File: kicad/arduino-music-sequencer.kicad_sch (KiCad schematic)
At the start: 130 parts, among them U1 CD74HC4067M

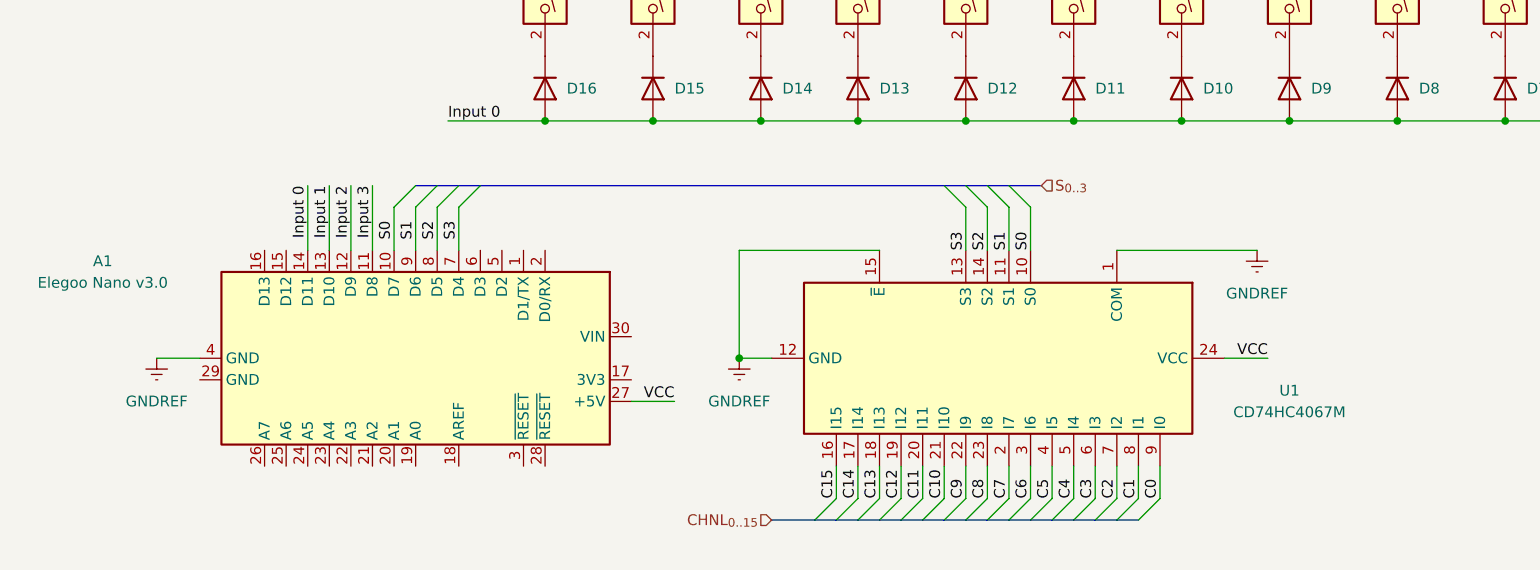
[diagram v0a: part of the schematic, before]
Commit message: Add files via upload
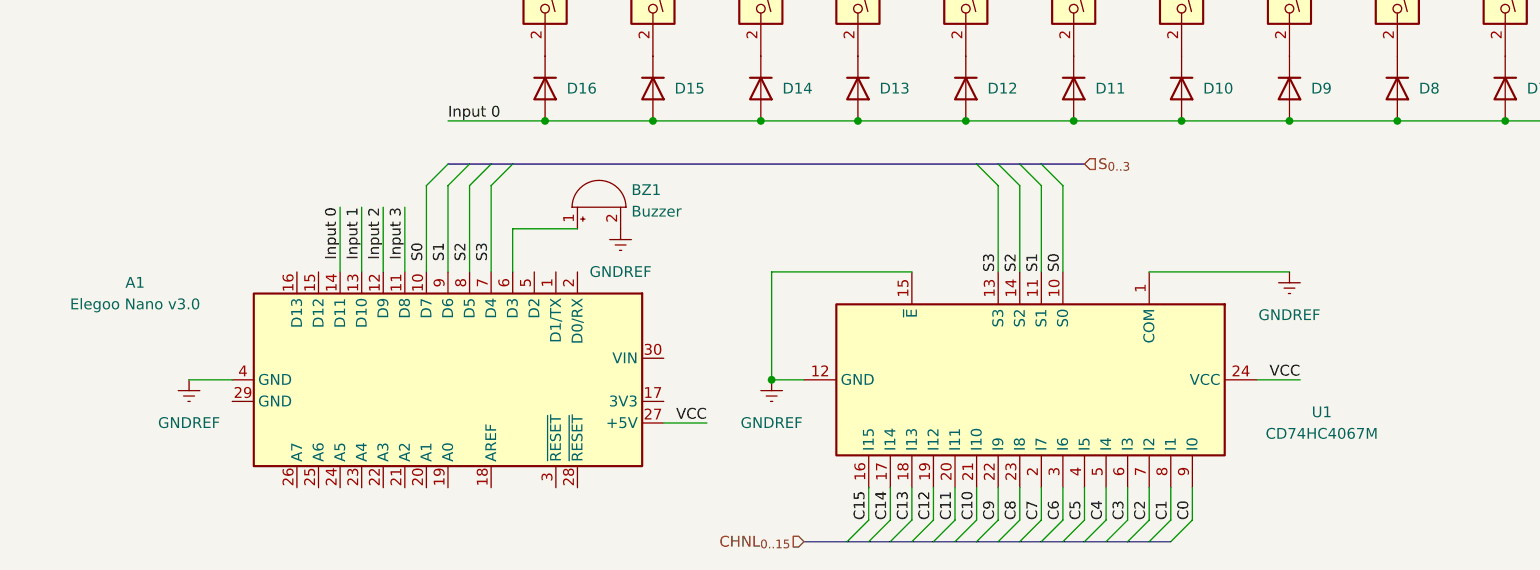
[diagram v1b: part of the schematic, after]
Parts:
- added BZ1: Buzzer, symbol Device:Buzzer
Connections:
- net GNDREF: now also BZ1.2 (-)
- net at A1.6 (D3): now also BZ1.1 (+)
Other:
- moved on the sheet: A1, U1
